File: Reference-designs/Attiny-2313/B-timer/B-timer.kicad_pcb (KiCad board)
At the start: 2 copper layers, 106 parts, among them J2 Conn_02x03_Odd_Even, SW1 SW_Push, SW2 SW_Push, SW3 SW_Push, U1 ATTINY2313-20MU

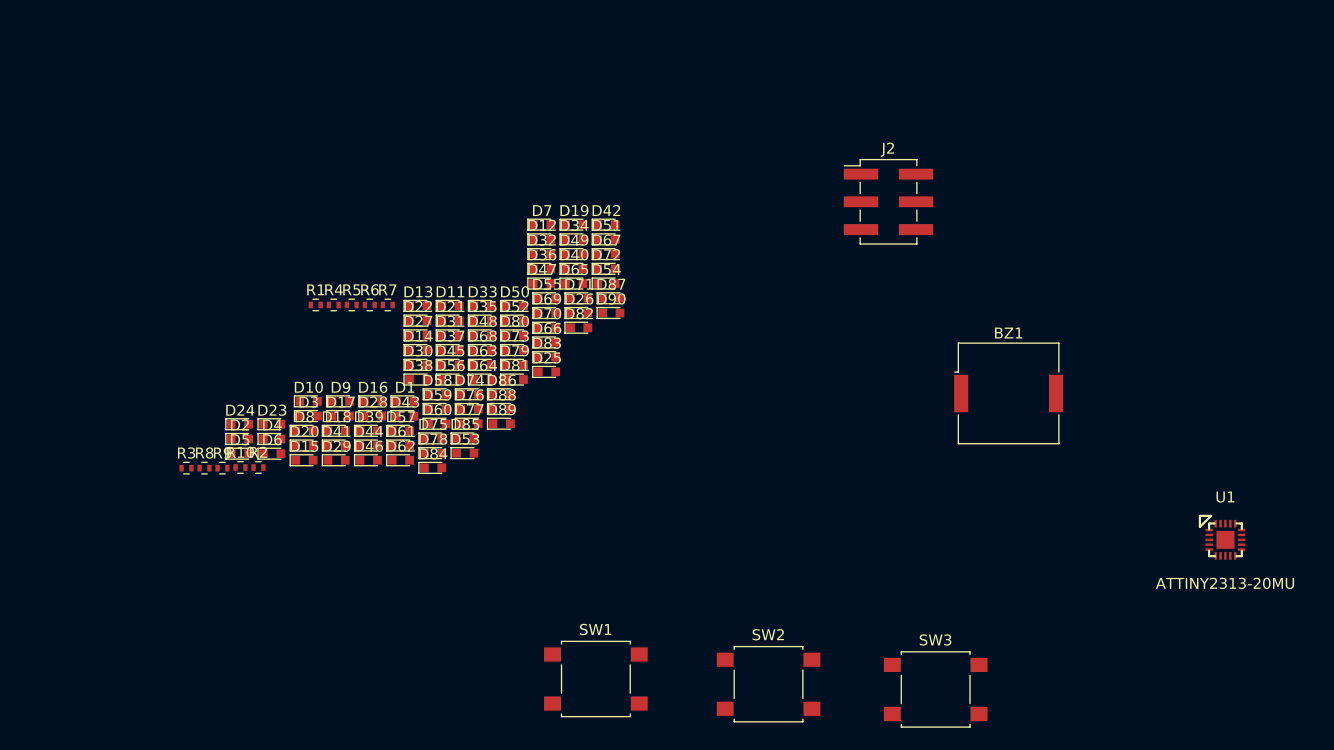
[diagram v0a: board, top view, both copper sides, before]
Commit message: First version layout
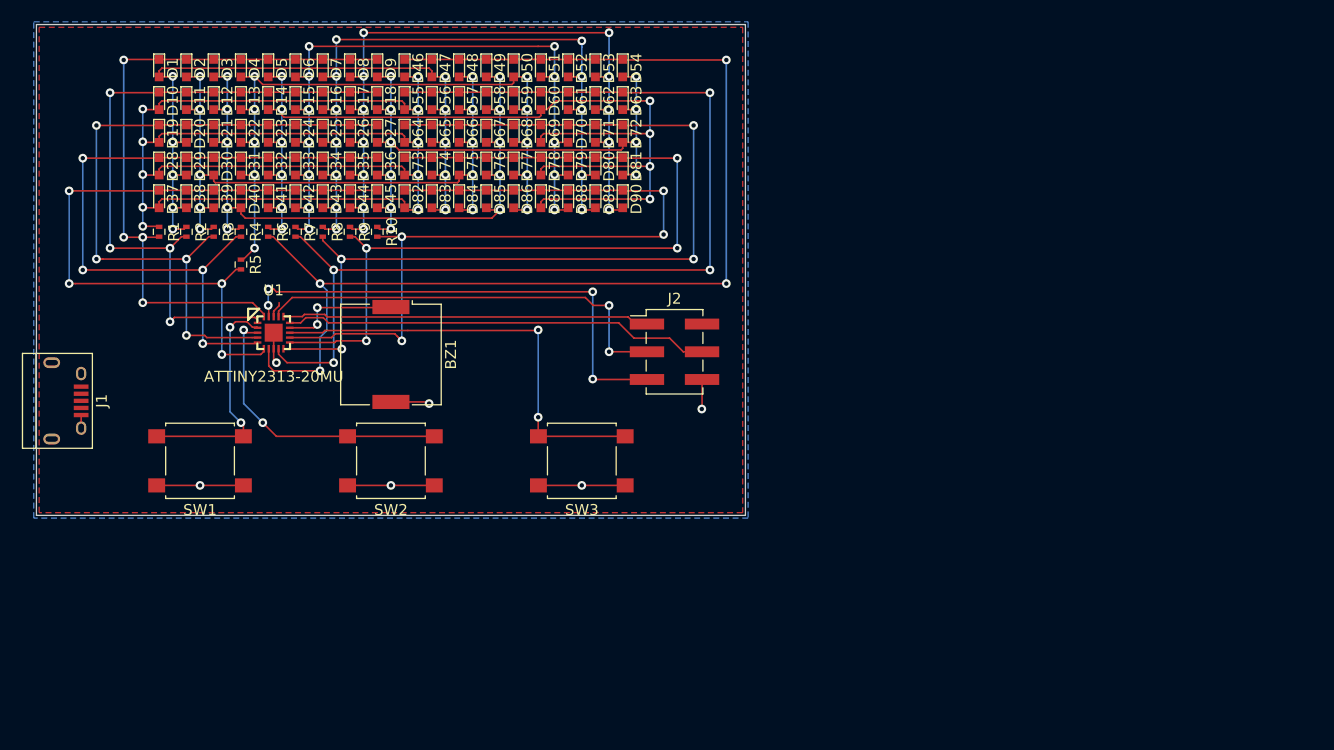
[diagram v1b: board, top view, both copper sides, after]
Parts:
- added J1: USB_B_Micro, Connectors:USB_Micro-B, F.Cu at (102.8, 89.5)
- moved U1 89.3 mm to (121.8, 83.2)
- moved BZ1 56.7 mm to (132.5, 85.2), turned to 270 degrees
- moved SW1 41.4 mm to (115.0, 95.0), turned to 180 degrees
- moved SW2 40.2 mm to (132.5, 95.0), turned to 180 degrees
- moved D19 39.0 mm to (111.2, 65.0), turned to 270 degrees
- moved SW3 38.6 mm to (150.0, 95.0), turned to 180 degrees
- moved D1 38.0 mm to (111.2, 59.0), turned to 270 degrees
- moved D62 37.5 mm to (151.2, 62.0), turned to 270 degrees
- moved D53 37.3 mm to (151.2, 59.0), turned to 270 degrees
- moved D46 36.1 mm to (133.8, 59.0), turned to 270 degrees
- moved D5 35.4 mm to (121.2, 59.0), turned to 270 degrees
- moved D6 35.4 mm to (123.8, 59.0), turned to 270 degrees
- moved D61 35.1 mm to (148.8, 62.0), turned to 270 degrees
- moved D2 34.3 mm to (113.8, 59.0), turned to 270 degrees
- moved D4 34.1 mm to (118.8, 59.0), turned to 270 degrees
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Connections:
- SW2 pad 1: Net-(SW2-Pad1) -> GND
- SW2 pad 2: GND -> Net-(SW2-Pad2)
- U1 pad 13: Net-(SW2-Pad1) -> Net-(SW3-Pad2)
- U1 pad 2: Net-(SW3-Pad2) -> Net-(SW1-Pad2)
- U1 pad 3: Net-(SW1-Pad2) -> Net-(SW2-Pad2)
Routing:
- net Net-(D10-Pad2): track 0.00 -> 132.2 mm, vias 0 -> 10
- net D5: track 0.00 -> 108.8 mm, vias 0 -> 4
- net Net-(D14-Pad2): track 0.00 -> 98.0 mm, vias 0 -> 10
- net D6: track 0.00 -> 97.9 mm, vias 0 -> 4
- net D7: track 0.00 -> 87.5 mm, vias 0 -> 4
- net D8: track 0.00 -> 79.3 mm, vias 0 -> 4
- net D9: track 0.00 -> 74.3 mm, vias 0 -> 4
- net Net-(D17-Pad2): track 0.00 -> 69.5 mm, vias 0 -> 12
- net Net-(D16-Pad2): track 0.00 -> 68.3 mm, vias 0 -> 12
- net Net-(D15-Pad2): track 0.00 -> 67.1 mm, vias 0 -> 12
- net Net-(D13-Pad2): track 0.00 -> 65.9 mm, vias 0 -> 10
- net Net-(D1-Pad2): track 0.00 -> 65.4 mm, vias 0 -> 10
- net D3: track 0.00 -> 64.9 mm, vias 0 -> 4
- net Net-(D12-Pad2): track 0.00 -> 63.9 mm, vias 0 -> 10
- net D4: track 0.00 -> 63.8 mm, vias 0 -> 4
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- added copper zone on F.Cu, net +5V
- added copper zone on B.Cu, net GND
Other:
- board outline added: 65 x 45 mm
- net class Default: clearance 0.2 -> 0.15; trace_width 0.25 -> 0.15
- rule trace_clearance: 0.2 -> 0.15
- rule trace_min: 0.2 -> 0.15
